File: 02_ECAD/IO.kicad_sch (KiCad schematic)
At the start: 126 parts, among them J1 3-1827253-6, J2 RFShield_OnePiece, J3 B10B-PHDSS, J4 Conn_Coaxial, Q5 2SK3018-TP, Q6 2SK3018-TP, Q7 2SK3018-TP, Q8 NX3020NAKS, Q9 NX3020NAKS, SW1 NANOT160AS, SW2 NANOT160AS, SW3 74404024010, U15 9FGV0241AKLF, U16 9FGV0241AKLF, U17 VSC8541XMV-02, U18 ESP-PSRAM32, U19 ESP32-PICO-D4, Y3 ABM3B-25.000MHZ-D4Y-T, Y4 ABM3B-25.000MHZ-D4Y-T, Y5 ABM3B-25.000MHZ-D4Y-T

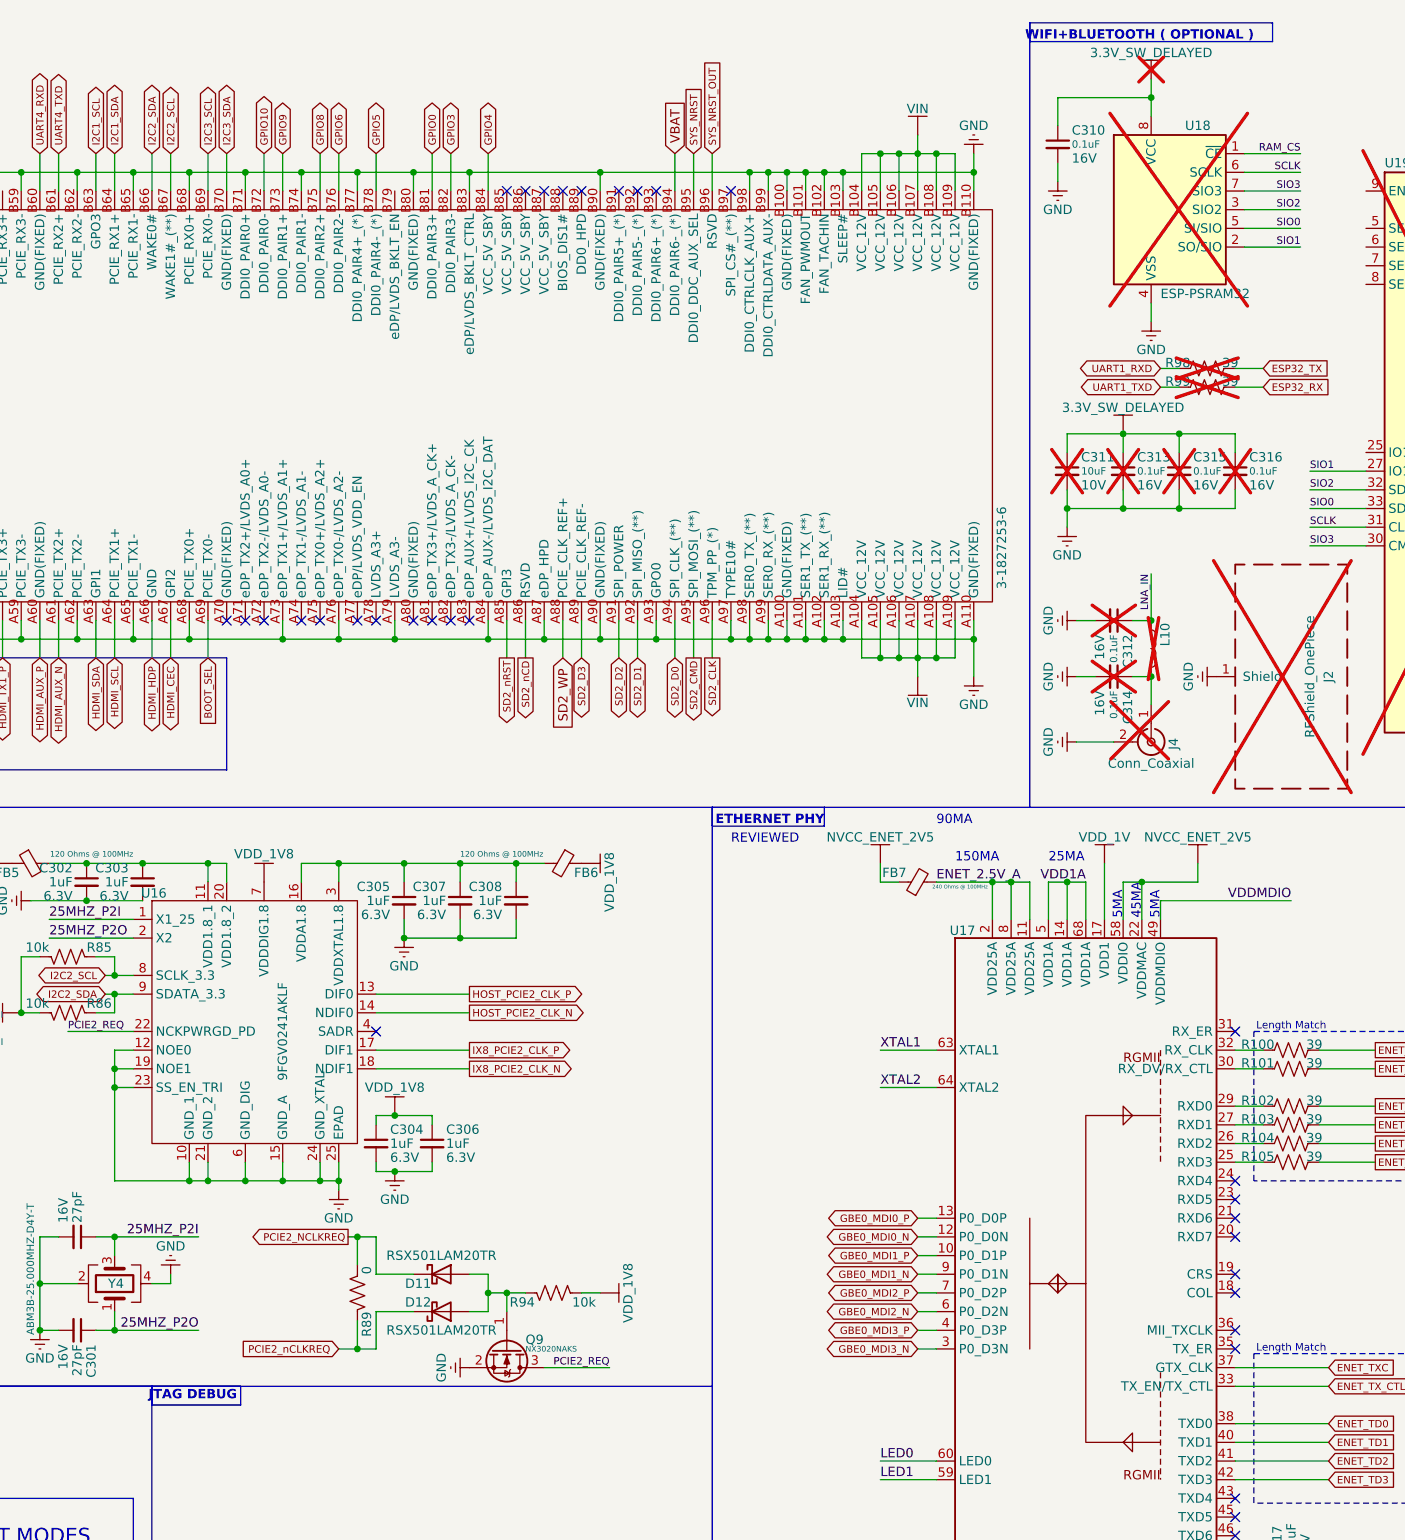
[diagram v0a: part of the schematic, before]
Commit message: Regular Update.
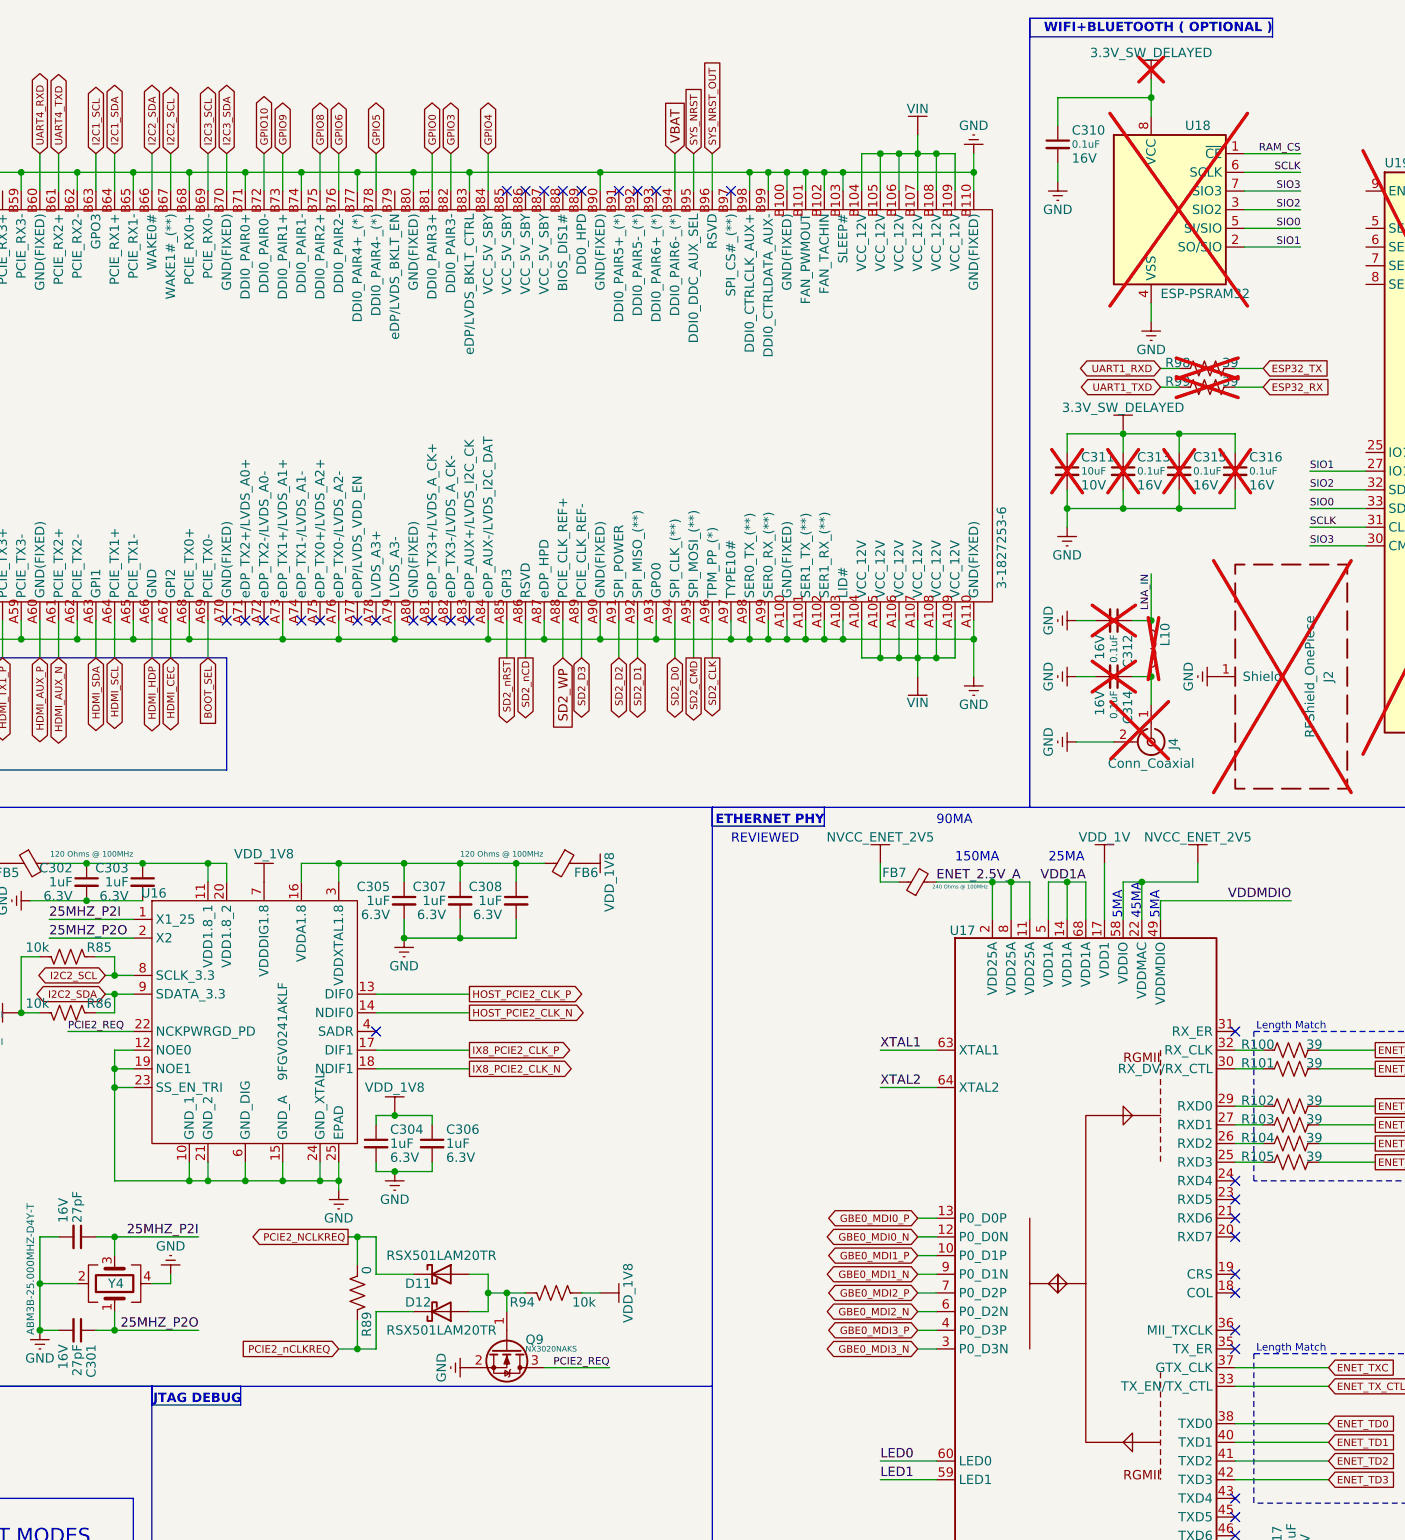
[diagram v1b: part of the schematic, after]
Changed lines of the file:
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@@
 	(polyline
 		(pts
-			(xy 307.34 12.7) (xy 307.34 119.38)
+			(xy 307.34 12.065) (xy 307.34 119.38)
 		)
 		(stroke
@@
 	)
 	(rectangle
-		(start 307.34 12.7)
-		(end 340.36 15.24)
+		(start 307.34 12.065)
+		(end 340.36 14.605)
 		(stroke
 			(width -0.0001)
@@
 	(text "WIFI+BLUETOOTH ( OPTIONAL )"
 		(exclude_from_sim no)
-		(at 337.82 15.24 0)
+		(at 340.36 14.224 0)
 		(effects
 			(font
@@
 	(text "JTAG DEBUG"
 		(exclude_from_sim no)
-		(at 199.517 200.152 0)
+		(at 200.152 200.66 0)
 		(effects
 			(font
@@
 		(shape bidirectional)
 		(at 233.68 30.48 90)
-		(fields_autoplaced yes)
 		(effects
 			(font
@@
 		)
 		(property "Intersheetrefs" "${INTERSHEET_REFS}"
-			(at 235.54 30.48 90)
+			(at 233.68 24.384 90)
 			(effects
 				(font
